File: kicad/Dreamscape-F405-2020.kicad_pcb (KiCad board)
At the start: 2 copper layers, 26.9 x 26.9 mm, 0 parts

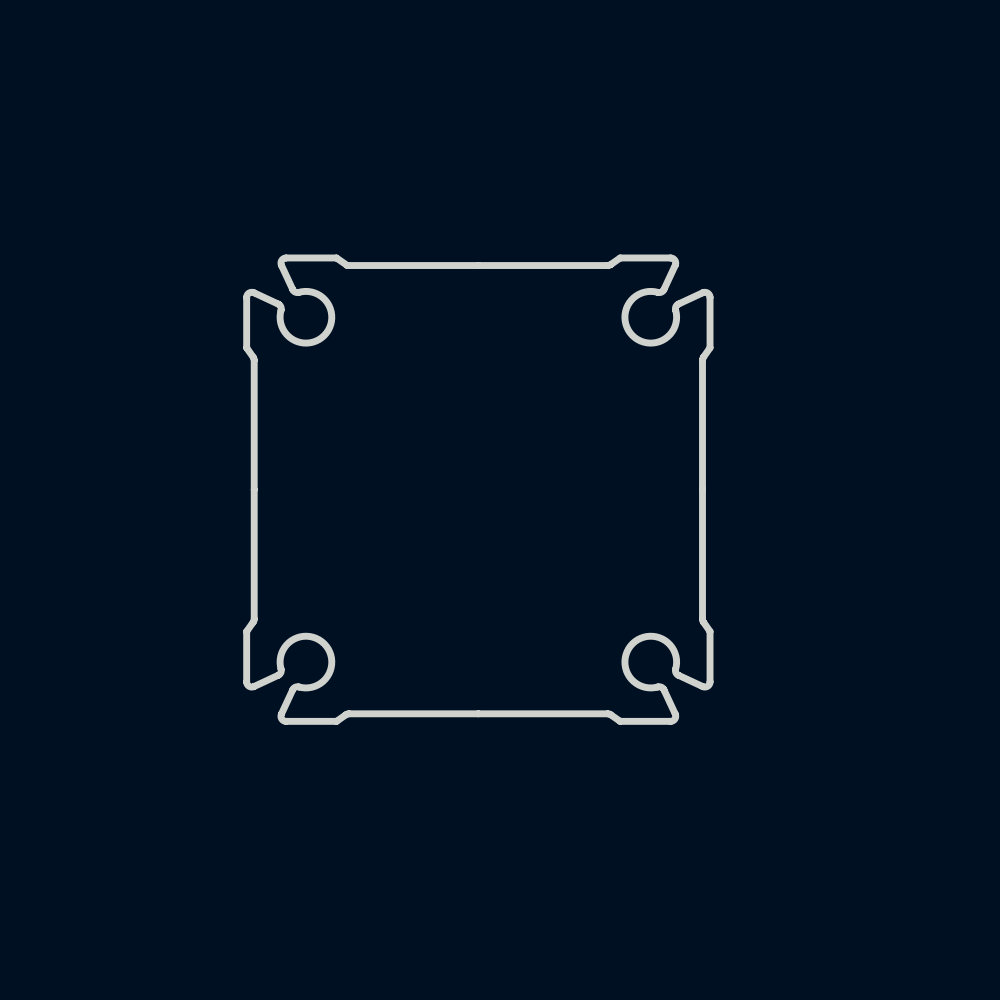
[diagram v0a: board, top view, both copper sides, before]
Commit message: journal
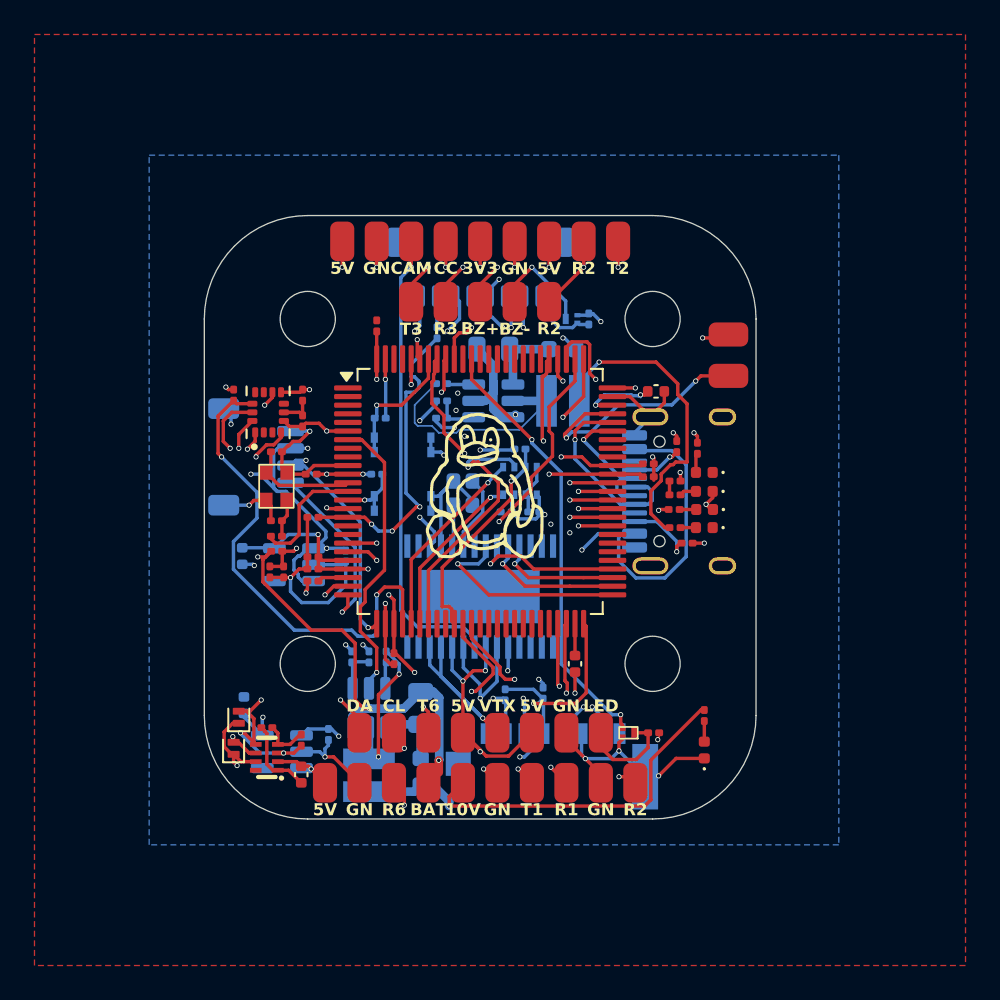
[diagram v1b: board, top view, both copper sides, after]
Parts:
- added C1: 4.7uF 50v, Capacitor_SMD:C_0805_2012Metric, B.Cu at (36.6, 52.6)
- added C10: 4.7uF, Capacitor_SMD:C_0402_1005Metric, F.Cu at (29.6, 56.4)
- added C11: 22uF, Capacitor_SMD:C_0402_1005Metric, B.Cu at (26.2, 43.8)
- added C12: 100n, Capacitor_SMD:C_0201_0603Metric, F.Cu at (29.7, 35.9)
- added C13: 100n, Capacitor_SMD:C_0201_0603Metric, B.Cu at (43.1, 41.2)
- added C14: 100n, Capacitor_SMD:C_0201_0603Metric, F.Cu at (29.7, 34.4)
- added C15: 100n, Capacitor_SMD:C_0201_0603Metric, B.Cu at (41.5, 41.2)
- added C16: 100n, Capacitor_SMD:C_0201_0603Metric, B.Cu at (43.6, 51.7)
- added C17: 100n, Capacitor_SMD:C_0201_0603Metric, F.Cu at (30.3, 43.8)
- added C18: 2.2uF, Capacitor_SMD:C_0402_1005Metric, F.Cu at (45.5, 50.0)
- added C19: 100n, Capacitor_SMD:C_0201_0603Metric, F.Cu at (34.0, 30.4)
- added C2: 4.7uF 50v, Capacitor_SMD:C_0805_2012Metric, B.Cu at (40.8, 31.8)
- added C20: 2.2uF, Capacitor_SMD:C_0402_1005Metric, F.Cu at (50.2, 34.2)
- added C21: 100n, Capacitor_SMD:C_0201_0603Metric, F.Cu at (30.3, 44.5)
- added C22: 20pF, Capacitor_SMD:C_0201_0603Metric, F.Cu at (28.2, 37.7)
- added C23: 100n, Capacitor_SMD:C_0201_0603Metric, F.Cu at (27.8, 44.7)
- added C24: 20pF, Capacitor_SMD:C_0201_0603Metric, F.Cu at (28.2, 41.7)
- added C25: 100n, Capacitor_SMD:C_0201_0603Metric, F.Cu at (30.3, 41.5)
- added C26: 100n, Capacitor_SMD:C_0201_0603Metric, F.Cu at (35.0, 49.7)
- added C27: 100n, Capacitor_SMD:C_0201_0603Metric, F.Cu at (30.2, 39.0)
- added C3: 100n, Capacitor_SMD:C_0201_0603Metric, B.Cu at (31.2, 54.1)
- added C4: 22uF, Capacitor_SMD:C_0402_1005Metric, B.Cu at (26.3, 52.4)
- added C5: 100n, Capacitor_SMD:C_0201_0603Metric, B.Cu at (34.6, 49.6)
- added C6: 100n, Capacitor_SMD:C_0201_0603Metric, B.Cu at (37.8, 33.8)
- added C7: 22uF, Capacitor_SMD:C_0603_1608Metric, B.Cu at (36.6, 56.3)
- added C8: 22uF, Capacitor_SMD:C_0603_1608Metric, B.Cu at (44.8, 31.8)
- added C9: 100n, Capacitor_SMD:C_0201_0603Metric, B.Cu at (32.2, 43.8)
- added Card1: TF-021B-H265, lib:TF-SMD_TF-021B-H265, B.Cu at (44.1, 55.3)
- added D1: LED_1_Green, LED_SMD:LED_0402_1005Metric, F.Cu at (53.0, 38.9)
- added D2: LED_1_Green, LED_SMD:LED_0402_1005Metric, F.Cu at (53.0, 55.0)
- added D3: LED_1_Green, LED_SMD:LED_0402_1005Metric, F.Cu at (53.0, 42.1)
- added D4: RB161QS-40_C28646385, Diode_SMD:D_SOD-882, F.Cu at (26.0, 53.1)
- added D5: RB161QS-40_C28646385, Diode_SMD:D_SOD-882, F.Cu at (25.7, 54.9)
- added D6: LED_1_Green, LED_SMD:LED_0402_1005Metric, F.Cu at (53.0, 41.0)
- added D7: LED_1_Blue, LED_SMD:LED_0402_1005Metric, F.Cu at (53.0, 40.0)
- added G***: LOGO, logo:linuxpenguin, F.Cu at (40.0, 40.0)
- added H1: MountingHole, MountingHole:MountingHole_3.2mm_M3, F.Cu at (50.0, 30.0)
- added H2: MountingHole, MountingHole:MountingHole_3.2mm_M3, F.Cu at (50.0, 50.0)
- added H3: MountingHole, MountingHole:MountingHole_3.2mm_M3, F.Cu at (30.0, 50.0)
- added H4: MountingHole, MountingHole:MountingHole_3.2mm_M3, F.Cu at (30.0, 30.0)
- added J1: 5V, lib:small_pad, F.Cu at (54.4, 30.9)
- added J10: 5V, lib:small_pad, F.Cu at (35.0, 54.0)
- added J11: 5V, lib:small_pad, F.Cu at (35.0, 56.9)
- added J12: 5V, lib:small_pad, F.Cu at (38.0, 25.5)
- added J13: 5V, lib:small_pad, F.Cu at (38.0, 29.0)
- added J14: 5V, lib:small_pad, F.Cu at (37.0, 54.0)
- added J15: 5V, lib:small_pad, F.Cu at (37.0, 56.9)
- added J16: 5V, lib:small_pad, F.Cu at (40.0, 25.5)
- added J17: 5V, lib:small_pad, F.Cu at (40.0, 29.0)
- added J18: 5V, lib:small_pad, F.Cu at (39.0, 54.0)
- added J19: 5V, lib:small_pad, F.Cu at (39.0, 56.9)
- added J2: 5V, lib:small_pad, F.Cu at (54.4, 33.3)
- added J20: 5V, lib:small_pad, F.Cu at (42.0, 25.5)
- added J21: 5V, lib:small_pad, F.Cu at (42.0, 29.0)
- added J22: 5V, lib:small_pad, F.Cu at (41.0, 54.0)
- added J23: 5V, lib:small_pad, F.Cu at (41.0, 56.9)
- added J24: 5V, lib:small_pad, F.Cu at (44.0, 25.5)
- added J25: 5V, lib:small_pad, F.Cu at (44.0, 29.0)
- added J26: 5V, lib:small_pad, F.Cu at (43.0, 54.0)
- added J27: 5V, lib:small_pad, F.Cu at (43.0, 56.9)
- added J28: 5V, lib:small_pad, F.Cu at (46.0, 25.5)
- added J29: 5V, lib:small_pad, F.Cu at (45.0, 54.0)
- added J3: 5V, lib:small_pad, F.Cu at (32.0, 25.5)
- added J30: 5V, lib:small_pad, F.Cu at (45.0, 56.9)
- added J31: 5V, lib:small_pad, F.Cu at (48.0, 25.5)
- added J32: 5V, lib:small_pad, F.Cu at (47.0, 54.0)
- added J33: 5V, lib:small_pad, F.Cu at (47.0, 56.9)
- added J34: 5V, lib:small_pad, F.Cu at (49.0, 56.9)
- added J35: Conn_01x08_MountingPin, Connector_JST:JST_SHL_SM08B-SHLS-TF_1x08-1MP_P1.00mm_Horizontal, B.Cu at (40.0, 27.0)
- added J36: Conn_01x04_MountingPin, Connector_JST:JST_SH_SM04B-SRSS-TB_1x04-1MP_P1.00mm_Horizontal, B.Cu at (27.0, 38.0)
- added J37: USB_C_Receptacle_USB2.0_16P, Connector_USB:USB_C_Receptacle_HRO_TYPE-C-31-M-12, B.Cu at (53.0, 40.0)
- added J4: 5V, lib:small_pad, F.Cu at (31.0, 56.9)
- added J5: 5V, lib:small_pad, F.Cu at (34.0, 25.5)
- added J6: 5V, lib:small_pad, F.Cu at (33.0, 54.0)
- added J7: 5V, lib:small_pad, F.Cu at (33.0, 56.9)
- added J8: 5V, lib:small_pad, F.Cu at (36.0, 25.5)
- added J9: 5V, lib:small_pad, F.Cu at (36.0, 29.0)
- added L1: XRTC303020D4R7MBCA, lib:IND-SMD_L3.0-W3.0_AFE303020S, B.Cu at (33.6, 56.5)
- added L2: XRTC303020D4R7MBCA, lib:IND-SMD_L3.0-W3.0_AFE303020S, B.Cu at (44.8, 34.8)
- added Q1: AP1606, lib:DFN-3L_L1.0-W0.6-P0.65-BR, F.Cu at (48.6, 54.0)
- added Q2: AP1606, lib:DFN-3L_L1.0-W0.6-P0.65-BR, B.Cu at (45.3, 30.0)
- added R1: 510R, Resistor_SMD:R_0201_0603Metric, F.Cu at (52.6, 37.5)
- added R10: 510R, Resistor_SMD:R_0201_0603Metric, F.Cu at (51.2, 41.0)
- added R11: 10k, Resistor_SMD:R_0201_0603Metric, F.Cu at (25.7, 34.4)
- added R12: 10k, Resistor_SMD:R_0201_0603Metric, B.Cu at (42.3, 37.5)
- added R13: 10k, Resistor_SMD:R_0201_0603Metric, B.Cu at (41.5, 51.8)
- added R14: 5.1k, Resistor_SMD:R_0201_0603Metric, F.Cu at (49.8, 39.1)
- added R15: 5.1k, Resistor_SMD:R_0201_0603Metric, F.Cu at (49.8, 38.4)
- added R16: 10k, Resistor_SMD:R_0201_0603Metric, B.Cu at (34.0, 39.0)
- added R17: 10k, Resistor_SMD:R_0201_0603Metric, B.Cu at (34.2, 35.8)
- added R18: 100k, Resistor_SMD:R_0201_0603Metric, F.Cu at (28.2, 43.5)
- added R19: 10k, Resistor_SMD:R_0201_0603Metric, F.Cu at (28.6, 44.7)
- added R2: 100k, Resistor_SMD:R_0201_0603Metric, B.Cu at (33.6, 49.6)
- added R20: 1k, Resistor_SMD:R_0201_0603Metric, B.Cu at (37.5, 30.8)
- added R21: 1k, Resistor_SMD:R_0201_0603Metric, F.Cu at (28.2, 42.6)
- added R22: 75R, Resistor_SMD:R_0201_0603Metric, F.Cu at (51.3, 39.4)
- added R23: 75R, Resistor_SMD:R_0201_0603Metric, F.Cu at (51.3, 40.2)
- added R24: 510R, Resistor_SMD:R_0201_0603Metric, F.Cu at (30.3, 45.2)
- added R25: 2.4k, Resistor_SMD:R_0201_0603Metric, F.Cu at (50.1, 54.0)
- added R26: 100k, Resistor_SMD:R_0201_0603Metric, B.Cu at (46.3, 30.0)
- added R27: 5.1k, Resistor_SMD:R_0201_0603Metric, F.Cu at (51.4, 37.4)
- added R28: 5.1k, Resistor_SMD:R_0201_0603Metric, F.Cu at (52.0, 43.0)
- added R3: 6.49k, Resistor_SMD:R_0201_0603Metric, B.Cu at (32.6, 49.6)
- added R4: 100k, Resistor_SMD:R_0201_0603Metric, B.Cu at (37.8, 35.8)
- added R5: 13.7k, Resistor_SMD:R_0201_0603Metric, B.Cu at (37.8, 34.8)
- added R6: 100k, Resistor_SMD:R_0201_0603Metric, F.Cu at (29.6, 54.4)
- added R7: 39k, Resistor_SMD:R_0201_0603Metric, F.Cu at (27.6, 53.7)
- added R8: 7.5k, Resistor_SMD:R_0201_0603Metric, F.Cu at (53.0, 53.0)
- added R9: 7.5k, Resistor_SMD:R_0201_0603Metric, F.Cu at (51.3, 42.1)
- added U1: TLV75733PDBV, Package_TO_SOT_SMD:SOT-23-5, B.Cu at (28.5, 55.1)
- added U11: TS2306A 240GF MSM 9_C2976675, lib:SW-SMD_4P-L3.0-W2.0-P0.85-LS3.5, B.Cu at (35.5, 40.7)
- added U12: TS2306A 240GF MSM 9_C2976675, lib:SW-SMD_4P-L3.0-W2.0-P0.85-LS3.5, B.Cu at (35.5, 37.3)
- added U2: LMR51430, Package_TO_SOT_SMD:SOT-23-6, B.Cu at (33.6, 52.6)
- added U3: LMR51430, Package_TO_SOT_SMD:SOT-23-6, B.Cu at (40.8, 34.8)
- added U4: TPS2116DRLR, lib:SOT-583-8_L2.1-W1.6-P0.50-LS1.6-BL, F.Cu at (27.6, 55.4)
- added U5: TLV75733PDBV, Package_TO_SOT_SMD:SOT-23-5, B.Cu at (29.2, 44.2)
- added U6: ICM-42688-P, ICM_42688_P:PQFN50P300X250X97-14N, F.Cu at (27.7, 35.4)
- added U7: BMP280, Package_LGA:Bosch_LGA-8_2x2.5mm_P0.65mm_ClockwisePinNumbering, B.Cu at (42.3, 39.4)
- added U8: AT7456E, footprints:21-0108G_U28E-5_MXM, B.Cu at (40.0, 46.1)
- added U9: STM32F405VGTx, Package_QFP:LQFP-100_14x14mm_P0.5mm, F.Cu at (40.0, 40.0)
- added X1: X32258MOB4SI, lib:CRYSTAL-SMD_4P-L2.5-W2.0-BL-A, F.Cu at (28.2, 39.7)
- added Y1: 27MHz, Crystal:Crystal_SMD_2016-4Pin_2.0x1.6mm, B.Cu at (39.0, 40.1)
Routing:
- net GND: track 0.00 -> 110.2 mm, vias 0 -> 25
- net +3.3V: track 0.00 -> 91.5 mm, vias 0 -> 19
- net +5V_BUCK: track 0.00 -> 74.5 mm, vias 0 -> 6
- net +5V: track 0.00 -> 71.0 mm, vias 0 -> 14
- net +BATT: track 0.00 -> 61.6 mm, vias 0 -> 5
- net /Pads/R2: track 0.00 -> 59.1 mm, vias 0 -> 4
- net +5V_USB: track 0.00 -> 52.7 mm, vias 0 -> 2
- net /STM32/IMU_INT1: track 0.00 -> 51.6 mm, vias 0 -> 2
- net /STM32/IMU_INT2: track 0.00 -> 48.8 mm, vias 0 -> 2
- net /Pads/T2: track 0.00 -> 41.2 mm, vias 0 -> 2
- net SPI1.SCK: track 0.00 -> 38.7 mm, vias 0 -> 2
- net +10V: track 0.00 -> 37.6 mm, vias 0 -> 2
- net /Pads/R3: track 0.00 -> 35.2 mm, vias 0 -> 2
- net /Pads/T3: track 0.00 -> 33.5 mm, vias 0 -> 2
- net +3.3VA: track 0.00 -> 32.4 mm, vias 0 -> 3
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- added copper zone on In1.Cu, net +3.3V
- added copper zone on In3.Cu, net +5V
- added copper zone on B.Cu, net GND
- added copper zone on F.Cu, net GND
- added copper zone on In2.Cu, net GND
- added copper zone on In4.Cu, net GND
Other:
- board size 26.9 x 26.9 mm -> 32 x 35 mm
- copper layers 2 -> 6
- board text added: "10V"
- board text added: "3V3"
- board text added: "5V"
- board text added: "BAT"
- board text added: "BZ+"
- board text added: "BZ-"
- board text added: "CAM"
- board text added: "CC"
- board text added: "CL"
- board text added: "DA"
- board text added: "GN"
- board text added: "LED"
- board text added: "R1"
- board text added: "R2"
- board text added: "R3"
- board text added: "R6"
- board text added: "T1"
- board text added: "T2"
- board text added: "T3"
- board text added: "T6"
- board text added: "VTX"

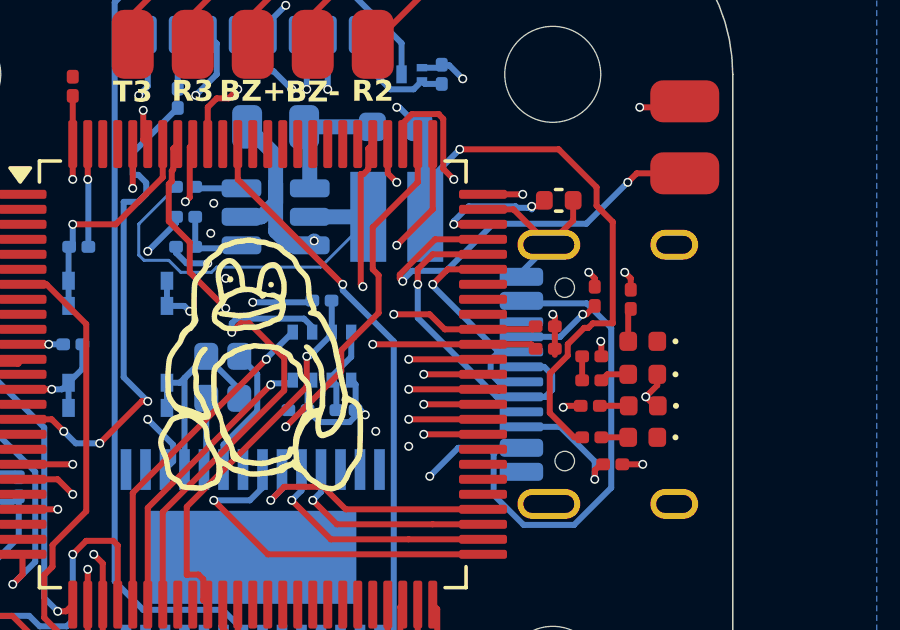
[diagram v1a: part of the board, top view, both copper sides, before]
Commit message: small changes
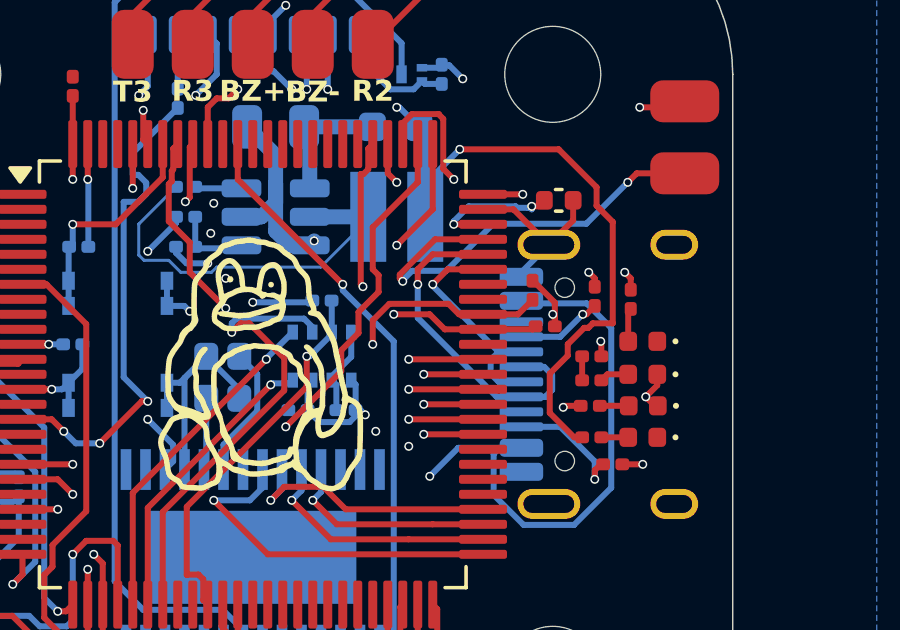
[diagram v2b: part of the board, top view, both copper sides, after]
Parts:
- moved R14 2.00 mm to (49.3, 37.2), turned to -90 degrees
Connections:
- U9 pad 65: /Pads/SDA -> unconnected-(U9-PC8-Pad65)
- U9 pad 67: unconnected-(U9-PA8-Pad67) -> /Pads/SDA
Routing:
- net /Pads/SDA: track 26.9 -> 28.1 mm
- net +3.3V: track 91.5 -> 92.4 mm
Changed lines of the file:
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@@
 			(layers "F.Cu" "F.Mask" "F.Paste")
 			(roundrect_rratio 0.25)
-			(net "/Pads/SDA")
+			(net "unconnected-(U9-PC8-Pad65)")
 			(pinfunction "PC8_65")
 			(pintype "bidirectional")
@@
 			(layers "F.Cu" "F.Mask" "F.Paste")
 			(roundrect_rratio 0.25)
-			(net "unconnected-(U9-PA8-Pad67)")
+			(net "/Pads/SDA")
 			(pinfunction "PA8_67")
 			(pintype "bidirectional")
@@
 	(footprint "Resistor_SMD:R_0201_0603Metric"
 		(layer "F.Cu")
-		(at 49.75 39.15 180)
+		(at 49.325 37.2 -90)
 		(descr "Resistor SMD 0201 (0603 Metric), square (rectangular) end terminal, IPC-7351 nominal, (Body size source: https://www.vishay.com/docs/20052/crcw0201e3.pdf)")
 		(tags "resistor")
 		(property "Reference" "R14"
-			(at 0 -1.05 0)
+			(at 0 -1.05 90)
 			(layer "F.SilkS")
 			(hide yes)
@@
 		)
 		(property "Value" "5.1k"
-			(at 0 1.05 0)
+			(at 0 1.05 90)
 			(layer "F.Fab")
 			(effects
@@
 		)
 		(property "Datasheet" ""
-			(at 0 0 0)
+			(at 0 0 90)
 			(layer "F.Fab")
 			(hide yes)
@@
 		)
 		(property "Description" "Resistor"
-			(at 0 0 0)
+			(at 0 0 90)
 			(layer "F.Fab")
 			(hide yes)
@@
 		)
 		(property "KiLib_Generator" "SMD_2terminal_chip_molded"
-			(at 0 0 0)
+			(at 0 0 90)
 			(layer "F.SilkS")
 			(hide yes)
@@
 		)
 		(property "LCSC" "C270344"
-			(at 0 0 180)
+			(at 0 0 270)
 			(unlocked yes)
 			(layer "F.Fab")
@@
 		)
 		(property "MPN" "0201WMF5101TEE"
-			(at 0 0 180)
+			(at 0 0 270)
 			(unlocked yes)
 			(layer "F.Fab")
@@
 		)
 		(property "Manufacturer" "UNI-ROYAL"
-			(at 0 0 180)
+			(at 0 0 270)
 			(unlocked yes)
 			(layer "F.Fab")
@@
 		)
 		(fp_text user "${REFERENCE}"
-			(at 0 -0.680001 0)
+			(at 0 -0.680001 90)
 			(layer "F.Fab")
 			(effects
@@
 		)
 		(pad "" smd roundrect
-			(at -0.345 0 180)
+			(at -0.345 0 270)
 			(size 0.318 0.36)
 			(layers "F.Paste")
@@
 		)
 		(pad "" smd roundrect
-			(at 0.345 0 180)
+			(at 0.345 0 270)
 			(size 0.318 0.36)
 			(layers "F.Paste")
@@
 		)
 		(pad "1" smd roundrect
-			(at -0.32 0 180)
+			(at -0.32 0 270)
 			(size 0.46 0.4)
 			(layers "F.Cu" "F.Mask")
@@
 		)
 		(pad "2" smd roundrect
-			(at 0.32 0 180)
+			(at 0.32 0 270)
 			(size 0.46 0.4)
 			(layers "F.Cu" "F.Mask")
@@
 	)
 	(segment
+		(start 50.07 37.607964)
+		(end 49.342036 36.88)
+		(width 0.2)
+		(layer "F.Cu")
+		(net "+3.3V")
+	)
+	(segment
 		(start 32.325 39)
 		(end 31.1 39)
@@
 	)
 	(segment
-		(start 50.07 39.349999)
-		(end 50.07 39.15)
-		(width 0.2)
-		(layer "F.Cu")
-		(net "+3.3V")
-	)
-	(segment
 		(start 50.07 38.07)
 		(end 50 38)
@@
 	)
 	(segment
+		(start 49.342036 36.88)
+		(end 49.325 36.88)
+		(width 0.2)
+		(layer "F.Cu")
+		(net "+3.3V")
+	)
+	(segment
 		(start 34 32.325)
 		(end 34 30.72)
@@
 	)
 	(segment
-		(start 29.700001 36.234999)
-		(end 29.885 36.05)
+		(start 50.07 37.607964)
+		(end 50.07 38.4)
 		(width 0.2)
 		(layer "F.Cu")
@@
 	)
 	(segment
-		(start 50.07 39.15)
-		(end 50.07 38.4)
+		(start 29.700001 36.234999)
+		(end 29.885 36.05)
 		(width 0.2)
 		(layer "F.Cu")
@@
 	)
 	(segment
-		(start 49.28 39)
-		(end 49.43 39.15)
+		(start 44.555025 37.65)
+		(end 46.525001 37.65)
 		(width 0.2)
 		(layer "F.Cu")
@@
 	)
 	(segment
-		(start 33 53.2)
-		(end 33 54)
+		(start 46.875001 38)
+		(end 47.675 38)
 		(width 0.2)
 		(layer "F.Cu")
@@
 	)
 	(segment
-		(start 44 39)
-		(end 47.675 39)
+		(start 44 38.205025)
+		(end 44.555025 37.65)
 		(width 0.2)
 		(layer "F.Cu")
@@
 	)
 	(segment
-		(start 47.675 39)
-		(end 49.28 39)
+		(start 33 53.2)
+		(end 33 54)
+		(width 0.2)
+		(layer "F.Cu")
+		(net "/Pads/SDA")
+	)
+	(segment
+		(start 47.675 38)
+		(end 48.845 38)
 		(width 0.2)
 		(layer "F.Cu")
@@
 		(net "/Pads/SDA")
 	)
+	(segment
+		(start 46.525001 37.65)
+		(end 46.875001 38)
+		(width 0.2)
+		(layer "F.Cu")
+		(net "/Pads/SDA")
+	)
+	(segment
+		(start 48.845 38)
+		(end 49.325 37.52)
+		(width 0.2)
+		(layer "F.Cu")
+		(net "/Pads/SDA")
+	)
+	(segment
+		(start 44 39)
+		(end 44 38.205025)
+		(width 0.2)
+		(layer "F.Cu")
+		(net "/Pads/SDA")
+	)
 	(via
 		(at 44 39)
@@
 	)
 	(segment
-		(start 41.1 41.75)
-		(end 42.95 39.9)
+		(start 44 35.1)
+		(end 45.5 33.6)
 		(width 0.2)
 		(layer "F.Cu")
@@
 	)
 	(segment
-		(start 44.194548 37.954833)
+		(start 42.95 39.199381)
+		(end 43.525 38.624381)
+		(width 0.2)
+		(layer "F.Cu")
+		(net "/Blackbox/FLASH_CS")
+	)
+	(segment
+		(start 43.525 38.624381)
+		(end 43.525 37.925)
+		(width 0.2)
+		(layer "F.Cu")
+		(net "/Blackbox/FLASH_CS")
+	)
+	(segment
+		(start 44.194548 37.255452)
 		(end 44.194548 36.694548)
 		(width 0.2)
@@
 	)
 	(segment
-		(start 42.95 39.199381)
-		(end 44.194548 37.954833)
+		(start 44.194548 36.694548)
+		(end 44 36.5)
 		(width 0.2)
 		(layer "F.Cu")
@@
 	)
 	(segment
-		(start 44.194548 36.694548)
-		(end 44 36.5)
+		(start 43.525 37.925)
+		(end 44.194548 37.255452)
 		(width 0.2)
 		(layer "F.Cu")
@@
 	)
 	(segment
-		(start 44 35.1)
-		(end 45.5 33.6)
+		(start 41.1 41.75)
+		(end 42.95 39.9)
 		(width 0.2)
 		(layer "F.Cu")
